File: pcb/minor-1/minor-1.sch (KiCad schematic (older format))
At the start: 40 parts, among them J1 AudioJack2_SwitchT, SW1 SW_SPST, SW10 SW_SPST, SW11 SW_SPST, SW12 SW_SPST, SW13 SW_SPST, SW14 SW_SPST, SW15 SW_SPST, SW16 SW_SPST, SW17 SW_SPST, SW18 SW_SPDT, SW2 SW_SPST, SW3 SW_SPST, SW4 SW_SPST, SW5 SW_SPST, SW6 SW_SPST, SW7 SW_SPST, SW8 SW_SPST, SW9 SW_SPST, U1 ATtiny3216-M, U2 PAM8302AAS, U3 MCP4018-xxxxLT, U4 TPS613221ADBV

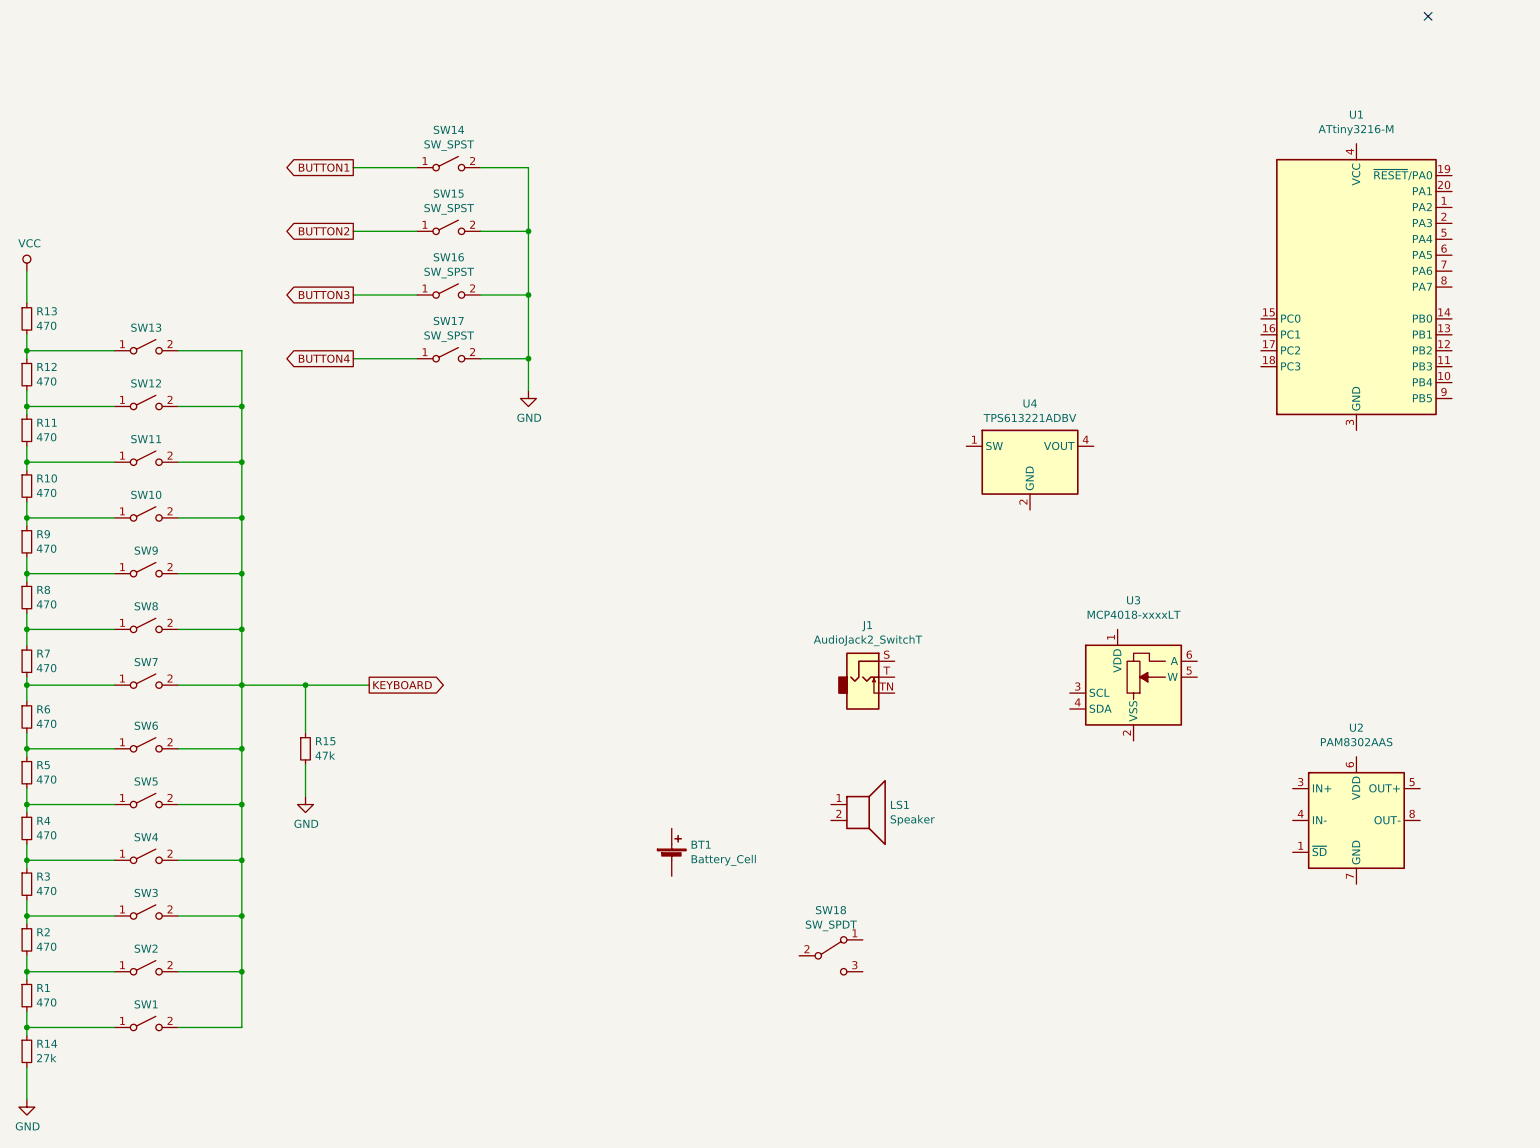
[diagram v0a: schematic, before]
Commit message: before silkscreen
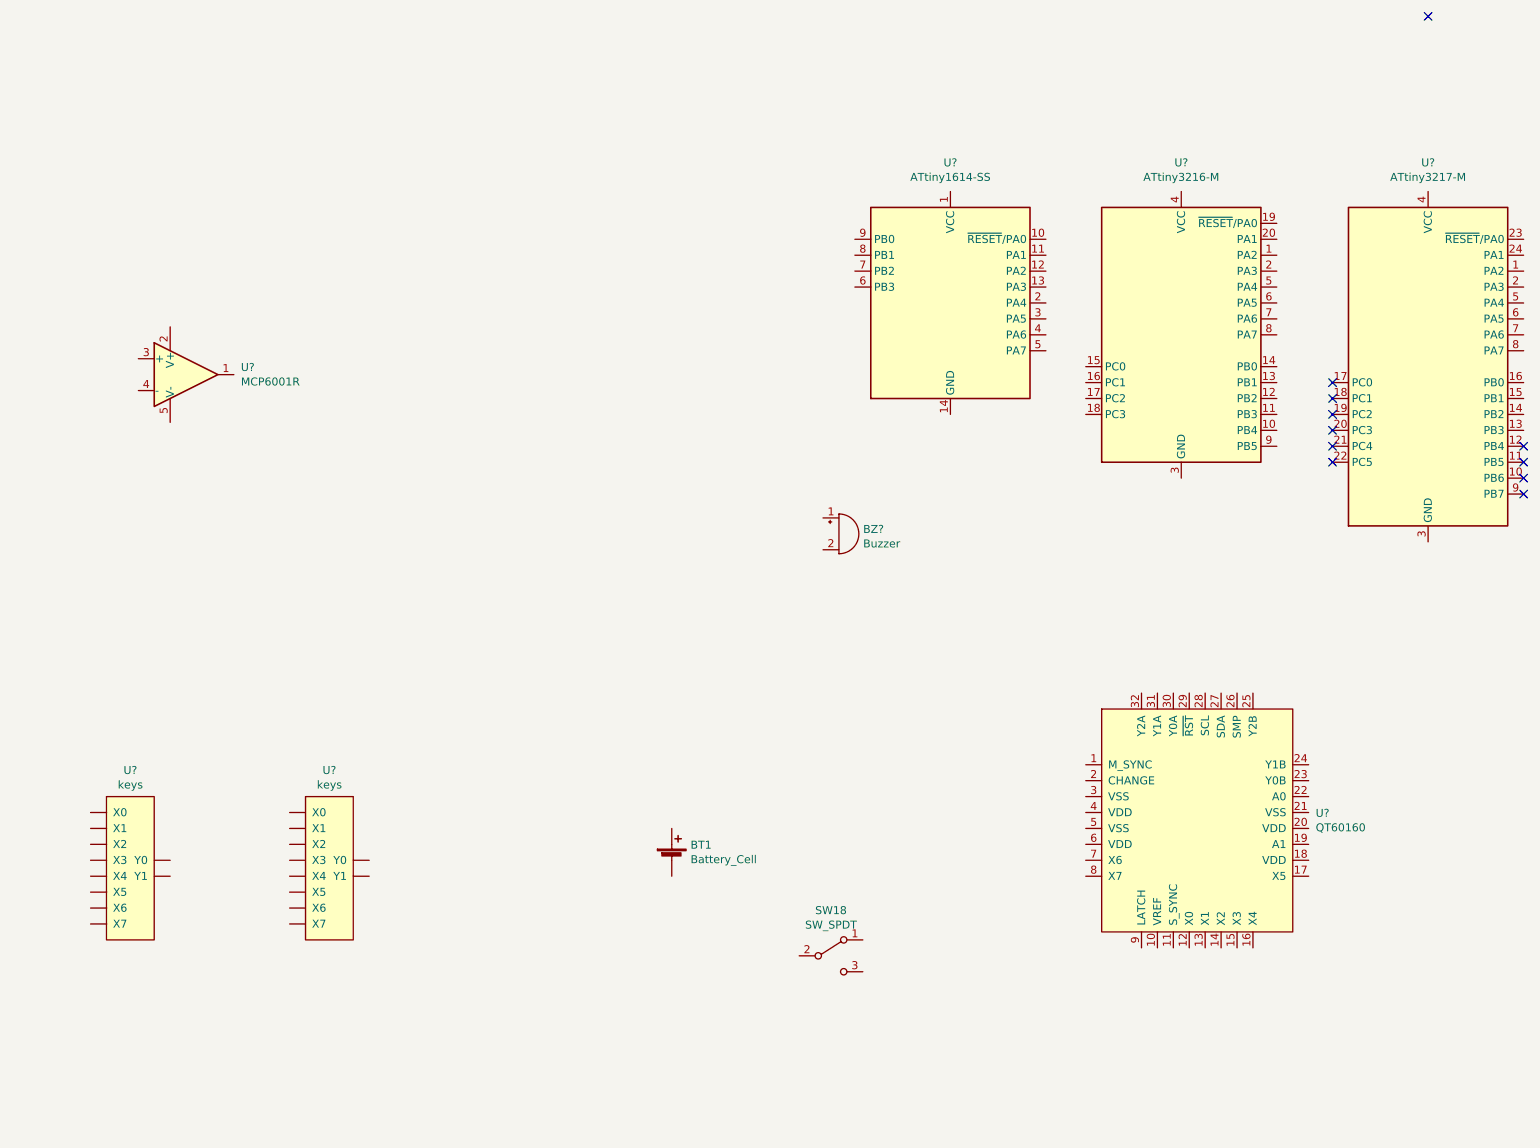
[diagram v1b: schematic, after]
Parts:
- removed J1: AudioJack2_SwitchT, SJ2-3592B-SMT-TR:CUI_SJ2-3592B-SMT-TR, symbol Connector:AudioJack2_SwitchT
- removed LS1: Speaker, CMS-15113-078S:SPKR_CMS-15113-078S, symbol Device:Speaker
- removed R1, R10, R11, R12, R13, R2, R3, R4, R5, R6, R7, R8, R9: 470, Resistors_SMD:R_0603, symbol Device:R_Small
- removed R14: 27k, Resistors_SMD:R_0603, symbol Device:R_Small
- removed R15: 47k, Resistors_SMD:R_0603, symbol Device:R_Small
- removed SW1, SW10, SW11, SW12, SW13, SW14, SW15, SW16, SW17, SW2, SW3, SW4, SW5, SW6, SW7, SW8, SW9: SW_SPST, EVQ-Q2B03W:EVQ-Q2B03W, symbol Switch:SW_SPST
- removed U1: ATtiny3216-M, Housings_DFN_QFN:UQFN-20-1EP_3x3mm_Pitch0.4mm, symbol MCU_Microchip_ATtiny:ATtiny3216-M
- removed U2: PAM8302AAS, Housings_SSOP:MSOP-8_3x3mm_Pitch0.65mm, symbol Amplifier_Audio:PAM8302AAS
- removed U3: MCP4018-xxxxLT, TO_SOT_Packages_SMD:SOT-363_SC-70-6, symbol Potentiometer_Digital:MCP4018-xxxxLT
- removed U4: TPS613221ADBV, TO_SOT_Packages_SMD:SOT-23-5, symbol Regulator_Switching:TPS613221ADBV
- added BZ?: Buzzer, symbol Device:Buzzer
- added U?: ATtiny1614-SS, Package_SO:SOIC-14_3.9x8.7mm_P1.27mm, symbol MCU_Microchip_ATtiny:ATtiny1614-SS
- added U?: MCP6001R, Package_TO_SOT_SMD:SOT-23-5, symbol Amplifier_Operational:MCP6001R
- added U? (x2): keys, symbol keyboard-13:keys
- added U?: QT60160, symbol QT60160:QT60160
- added U?: ATtiny3217-M, Package_DFN_QFN:QFN-24-1EP_4x4mm_P0.5mm_EP2.6x2.6mm, symbol MCU_Microchip_ATtiny:ATtiny3217-M
- added U?: ATtiny3216-M, Package_DFN_QFN:VQFN-20-1EP_3x3mm_P0.4mm_EP1.7x1.7mm, symbol MCU_Microchip_ATtiny:ATtiny3216-M
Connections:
- new net: U?.25 (GND), U?.3 (GND)
- new net: U?.21 (GND), U?.3 (GND)
- no-connect marks 1 -> 11
